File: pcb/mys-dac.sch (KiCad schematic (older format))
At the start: 39 parts, among them J1 OLED, J2 Conn_02x20_Odd_Even, J3 Conn_02x20_Odd_Even, J4 DAC, J5 IO, J6 CONSOLE, J7 SPDIF, J8 PWR_IN, U1 WM8805, U2 TLV62568DBV, U3 ISO7321C, Y1 12MHz

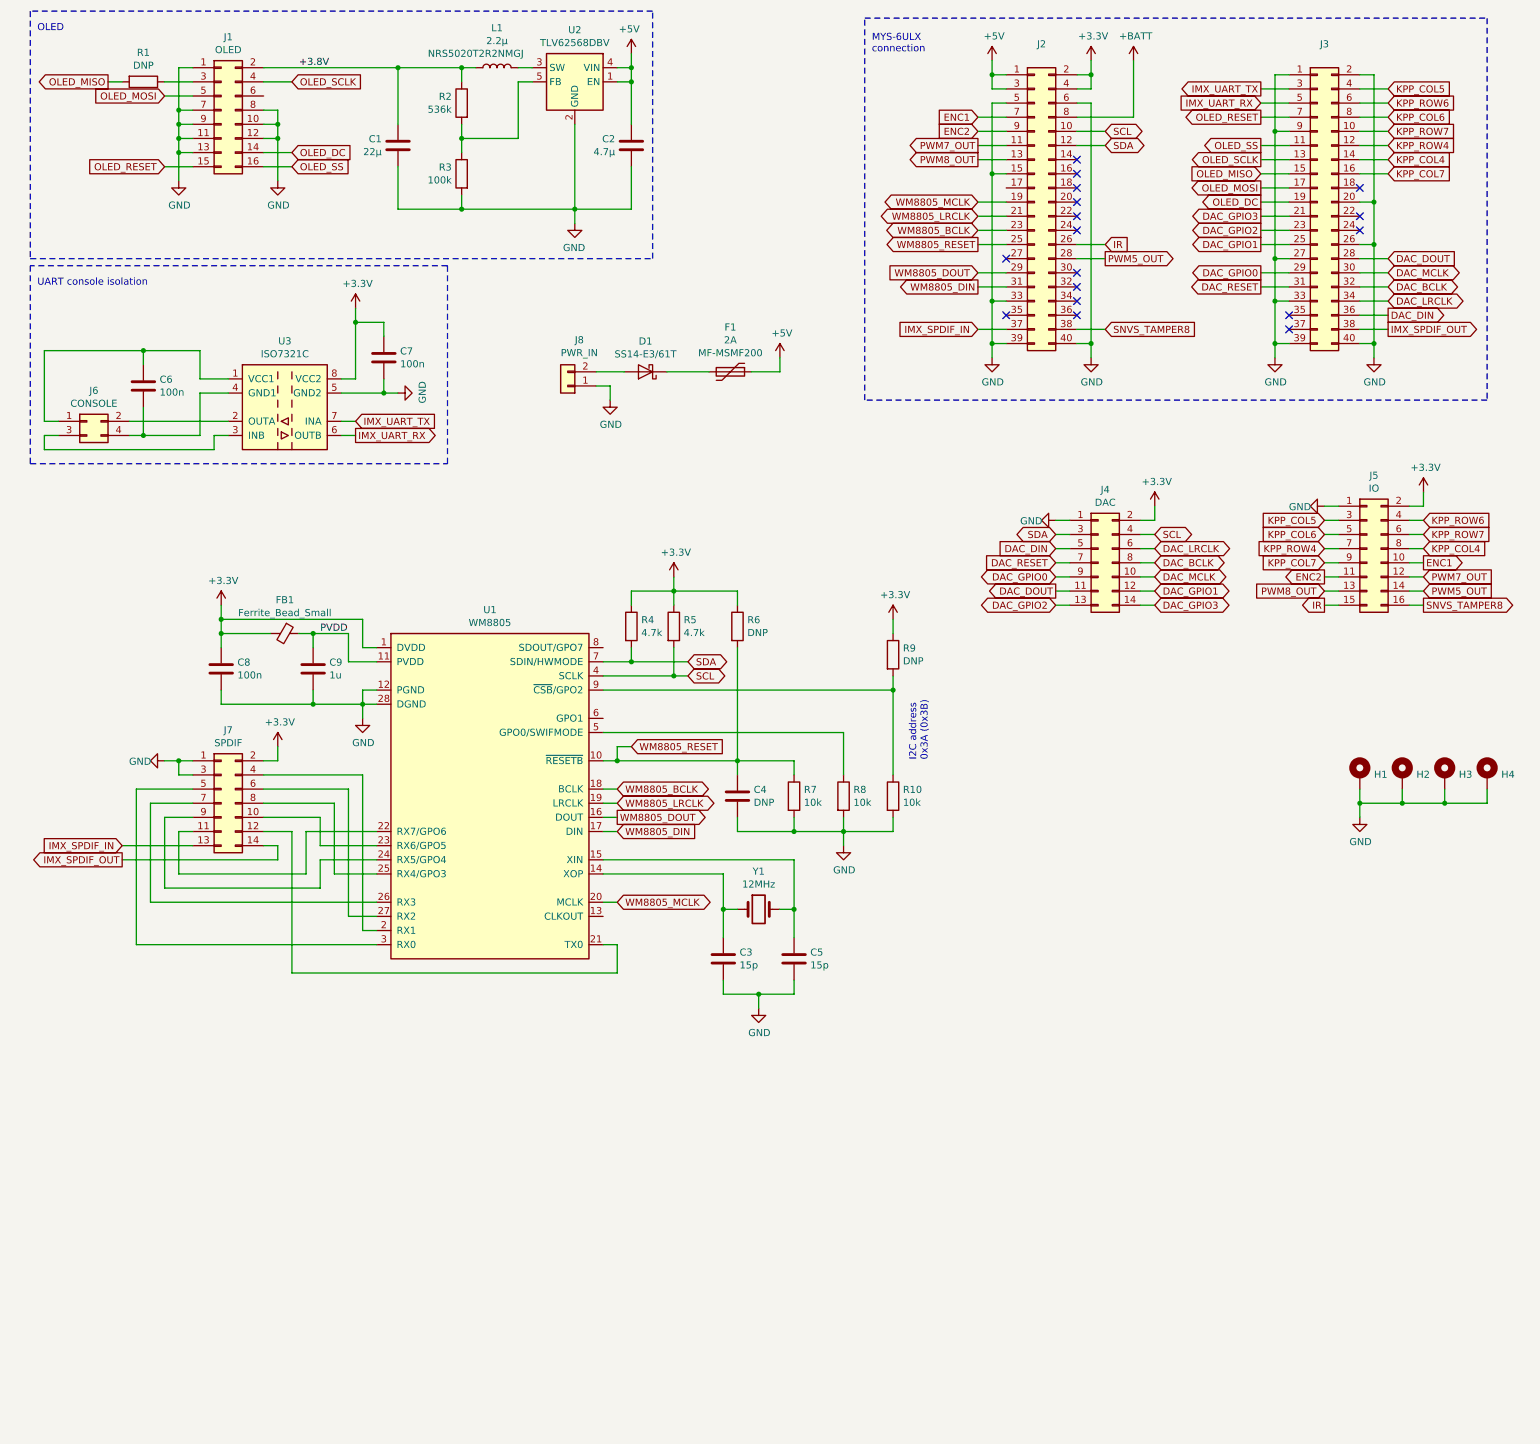
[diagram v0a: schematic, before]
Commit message: Done routing
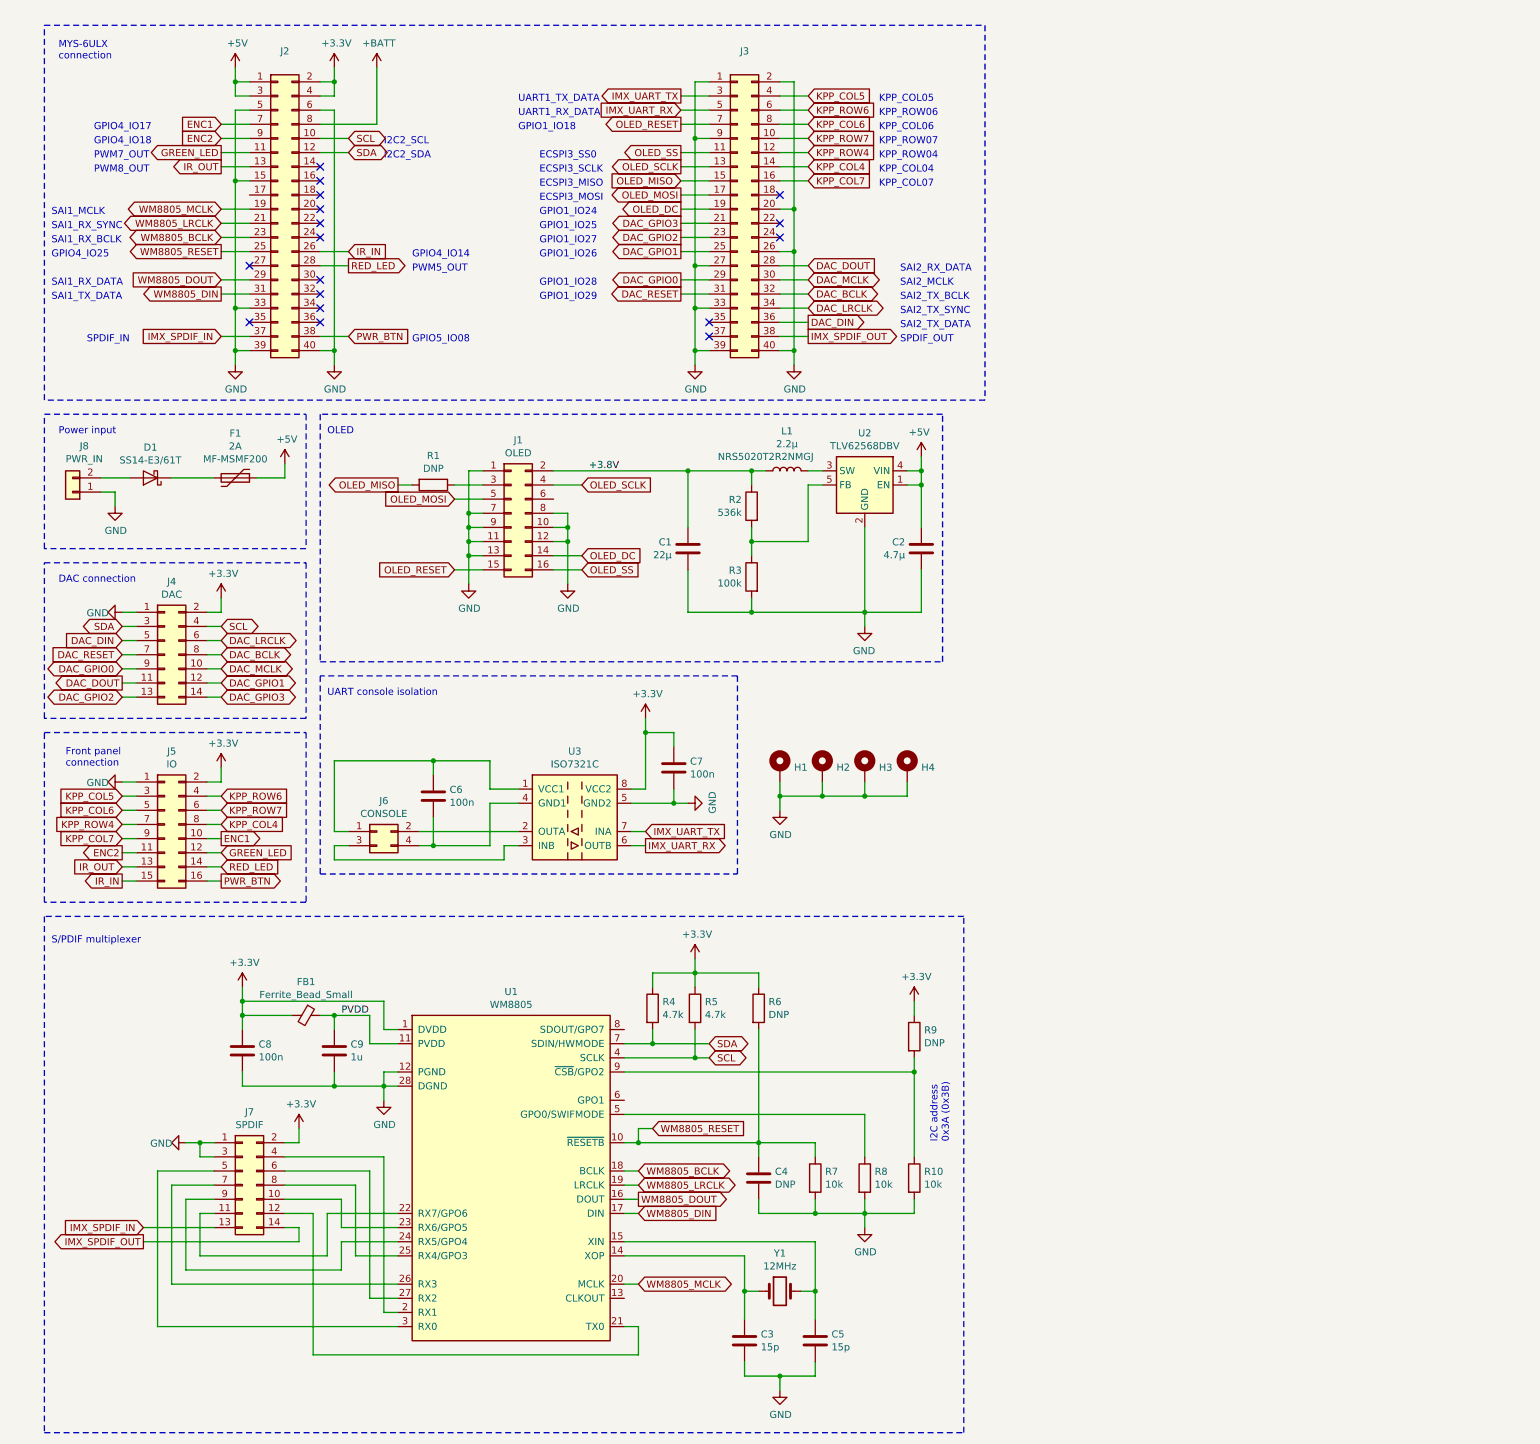
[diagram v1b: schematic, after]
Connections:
- net IR renamed IR_IN
- net PWM5_OUT renamed RED_LED
- net PWM7_OUT renamed GREEN_LED
- net PWM8_OUT renamed IR_OUT
- net SNVS_TAMPER8 renamed PWR_BTN
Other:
- note added: "DAC connection"
- note added: "ECSPI3_MISO"
- note added: "ECSPI3_MOSI"
- note added: "ECSPI3_SCLK"
- note added: "ECSPI3_SS0"
- note added: "Front panel\nconnection"
- note added: "GPIO1_IO18"
- note added: "GPIO1_IO24"
- note added: "GPIO1_IO25"
- note added: "GPIO1_IO26"
- note added: "GPIO1_IO27"
- note added: "GPIO1_IO28"
- note added: "GPIO1_IO29"
- note added: "GPIO4_IO14"
- note added: "GPIO4_IO17"
- note added: "GPIO4_IO18"
- note added: "GPIO4_IO25"
- note added: "GPIO5_IO08"
- note added: "I2C2_SCL"
- note added: "I2C2_SDA"
- note added: "KPP_COL04"
- note added: "KPP_COL05"
- note added: "KPP_COL06"
- note added: "KPP_COL07"
- note added: "KPP_ROW04"
- note added: "KPP_ROW06"
- note added: "KPP_ROW07"
- note added: "PWM5_OUT"
- note added: "PWM7_OUT"
- note added: "PWM8_OUT"
- note added: "Power input"
- note added: "S/PDIF multiplexer"
- note added: "SAI1_MCLK"
- note added: "SAI1_RX_BCLK"
- note added: "SAI1_RX_DATA"
- note added: "SAI1_RX_SYNC"
- note added: "SAI1_TX_DATA"
- note added: "SAI2_MCLK"
- note added: "SAI2_RX_DATA"
- note added: "SAI2_TX_BCLK"
- note added: "SAI2_TX_DATA"
- note added: "SAI2_TX_SYNC"
- note added: "SPDIF_IN"
- note added: "SPDIF_OUT"
- note added: "UART1_RX_DATA"
- note added: "UART1_TX_DATA"
- moved on the sheet: C1, C2, C3, C4, C5, C6, C7, C8, C9, D1, F1, FB1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
